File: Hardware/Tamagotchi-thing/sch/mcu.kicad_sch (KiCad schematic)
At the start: 30 parts, among them J2 Conn_01x04, J3 Conn_01x04, J6 USB_C_Receptacle_USB2.0, SW1 SW_Push, SW2 SW_Push, SW3 SW_Push, SW4 SW_MEC_5E, U1 USBLC6-2P6, U4 STM32L073RBTx, Y1 32768Hz - 12,5 pF

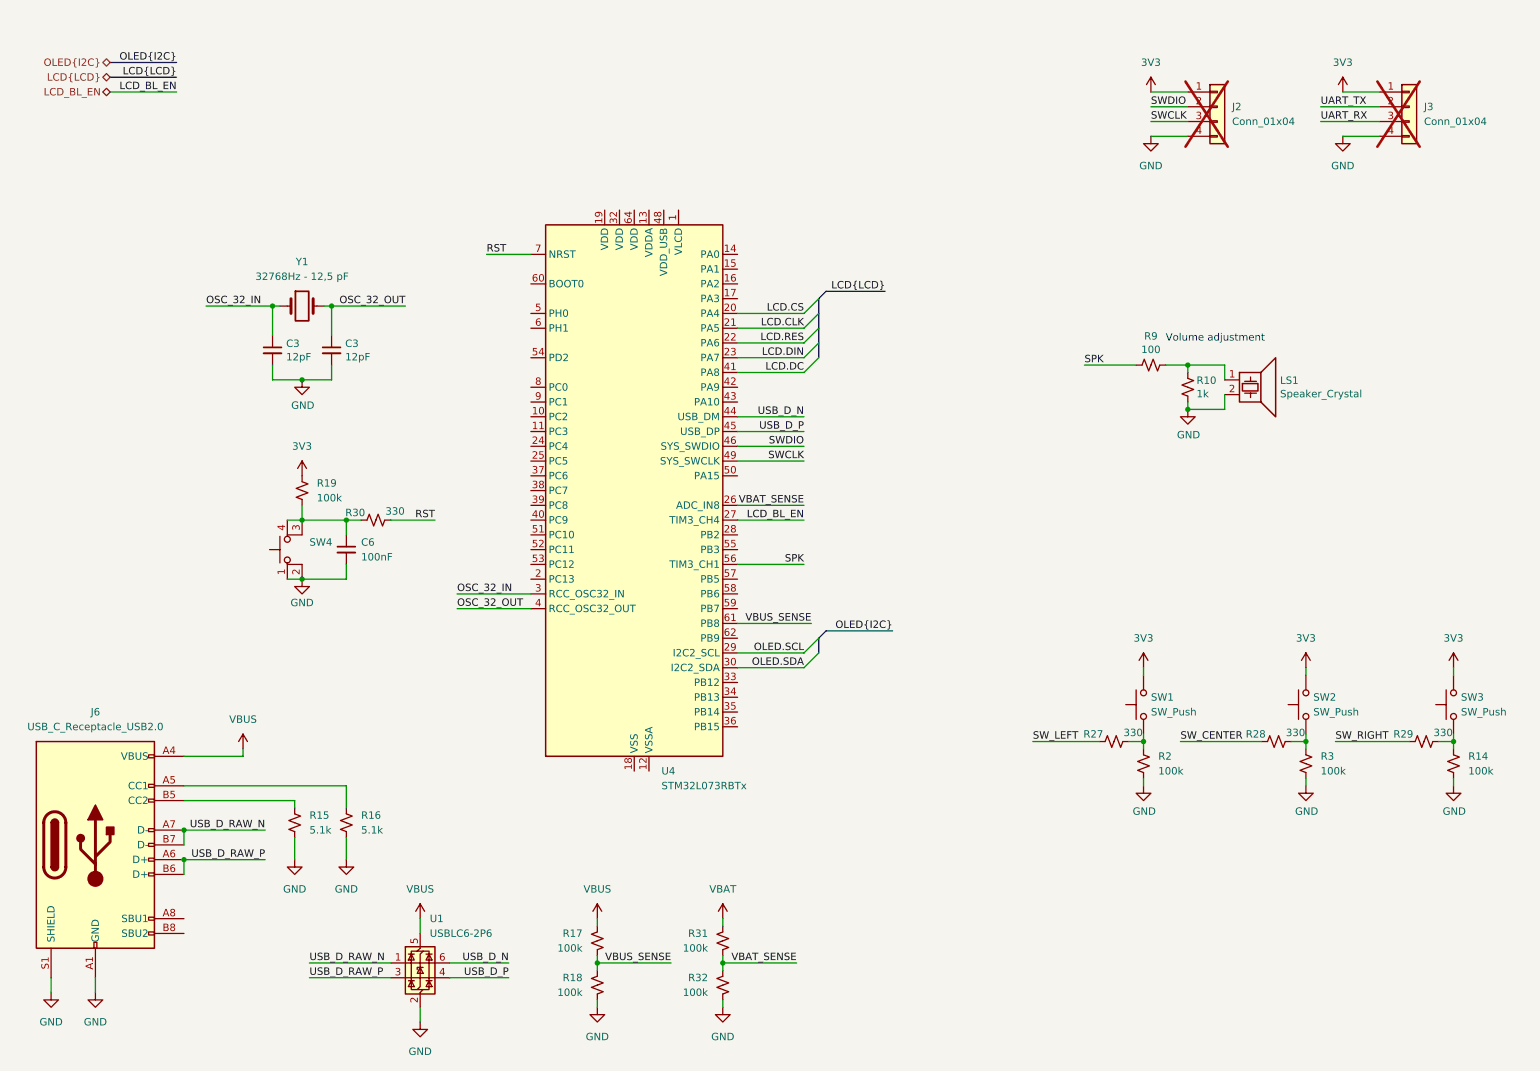
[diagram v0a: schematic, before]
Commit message: Schematic work
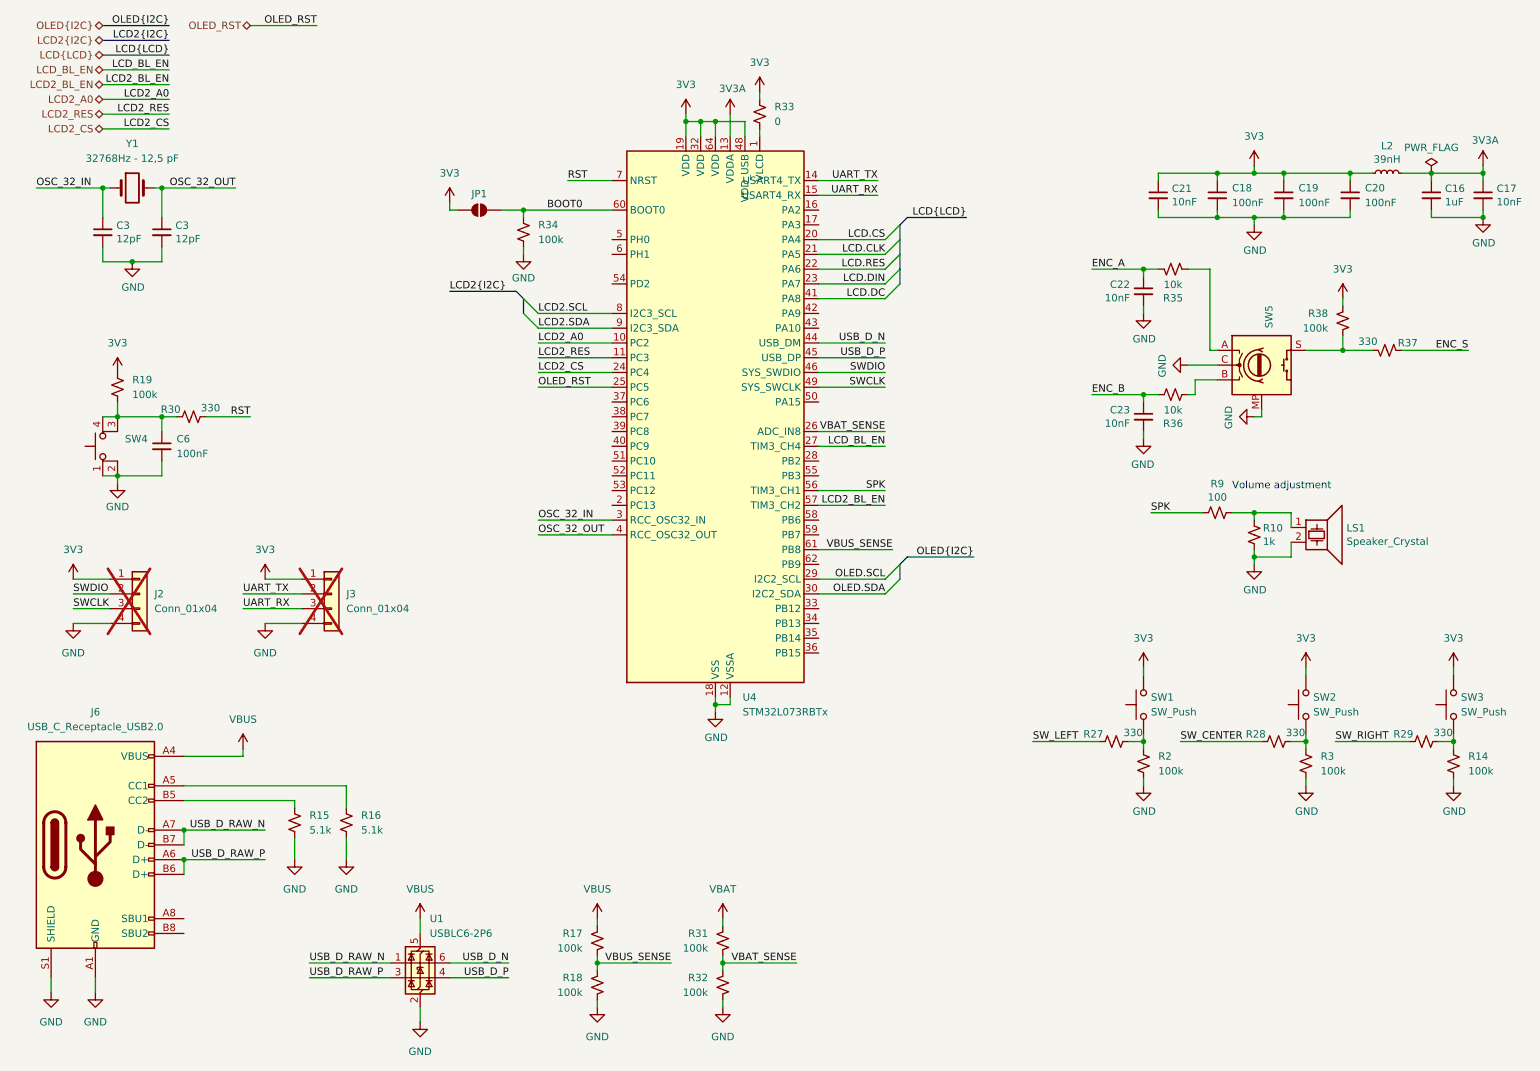
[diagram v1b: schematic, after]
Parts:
- added C16: 1uF, Capacitor_SMD:C_0603_1608Metric, symbol Device:C_Small
- added C17, C21, C22, C23: 10nF, Capacitor_SMD:C_0402_1005Metric, symbol Device:C_Small
- added C18, C19, C20: 100nF, Capacitor_SMD:C_0603_1608Metric, symbol Device:C_Small
- added JP1: SolderJumper_2_Open, Jumper:SolderJumper-2_P1.3mm_Open_Pad1.0x1.5mm, symbol Jumper:SolderJumper_2_Open
- added L2: 39nH, Inductor_SMD:L_0402_1005Metric, symbol Device:L_Small
- added R33: 0, symbol Device:R_Small_US
- added R34: 100k, Resistor_SMD:R_0603_1608Metric, symbol Device:R_Small_US
- added R35, R36: 10k, Resistor_SMD:R_0402_1005Metric, symbol Device:R_Small_US
- added R37: 330, symbol Device:R_Small_US
- added R38: 100k, symbol Device:R_Small_US
- added SW5: RotaryEncoder_Switch_MP, TamagotchiThing:SW-SMD_SIQ-02FVS3, symbol Device:RotaryEncoder_Switch_MP
- SW1, SW2, SW3: footprint (none) -> TamagotchiThing:Kailh_mouse_button; now left out of the parts list
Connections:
- net 3V3: now also U4.19 (VDD), U4.32 (VDD), U4.48 (VDD_USB), U4.64 (VDD), C18.1, C19.1, C20.1, C21.1, JP1.1 (A), L2.1, R33.1, R38.1
- net GND: now also U4.12 (VSSA), U4.18 (VSS), U4.31 (VSS), U4.47 (VSS), U4.63 (VSS), C16.2, C17.2, C18.2, C19.2, C20.2, C21.2, C22.2, C23.2, R34.2, SW5.C, SW5.MP
- net UART_RX: now also U4.15 (PA1)
- net UART_TX: now also U4.14 (PA0)
- net at U4.1 (VLCD): now also R33.2
- net LCD2_A0: now reaches U4.10 (PC2)
- net LCD2_RES: now reaches U4.11 (PC3)
- net 3V3A: now reaches U4.13 (VDDA)
- net 3V3A: now also C16.1, C17.1, L2.2
- net LCD2_CS: now reaches U4.24 (PC4)
- net OLED_RST: now reaches U4.25 (PC5)
- net LCD2_BL_EN: now reaches U4.57 (PB5)
- net BOOT0: now reaches U4.60 (BOOT0)
- net BOOT0: now also JP1.2 (B), R34.1
- net LCD2.SCL: now reaches U4.8 (PC0)
- net LCD2.SDA: now reaches U4.9 (PC1)
- new net: R35.1, SW5.A
- new net: R36.2, SW5.B
- new net: R37.2, R38.2, SW5.S
- new net ENC_A: C22.1, R35.2
- new net ENC_B: C23.1, R36.1
- new net ENC_S: R37.1
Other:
- moved on the sheet: C3, C6, J2, J3, LS1, R10, R19, R30, R9, SW4, U4, Y1
